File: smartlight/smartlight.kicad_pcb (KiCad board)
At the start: 2 copper layers, 43 x 37.5 mm, 22 parts, among them J1 Conn_01x06, J2 Conn_01x05, U1 ESP-12F

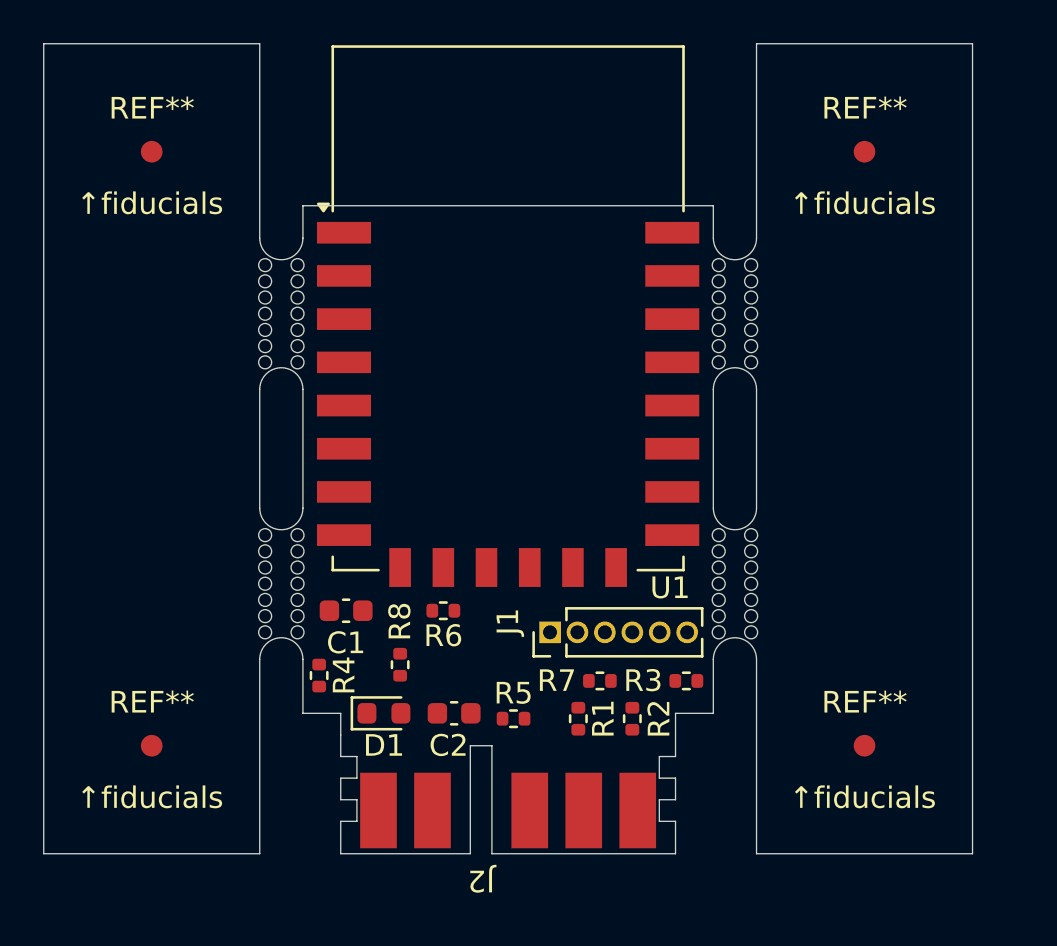
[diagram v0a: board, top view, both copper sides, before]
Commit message: before swapping pin snapshot
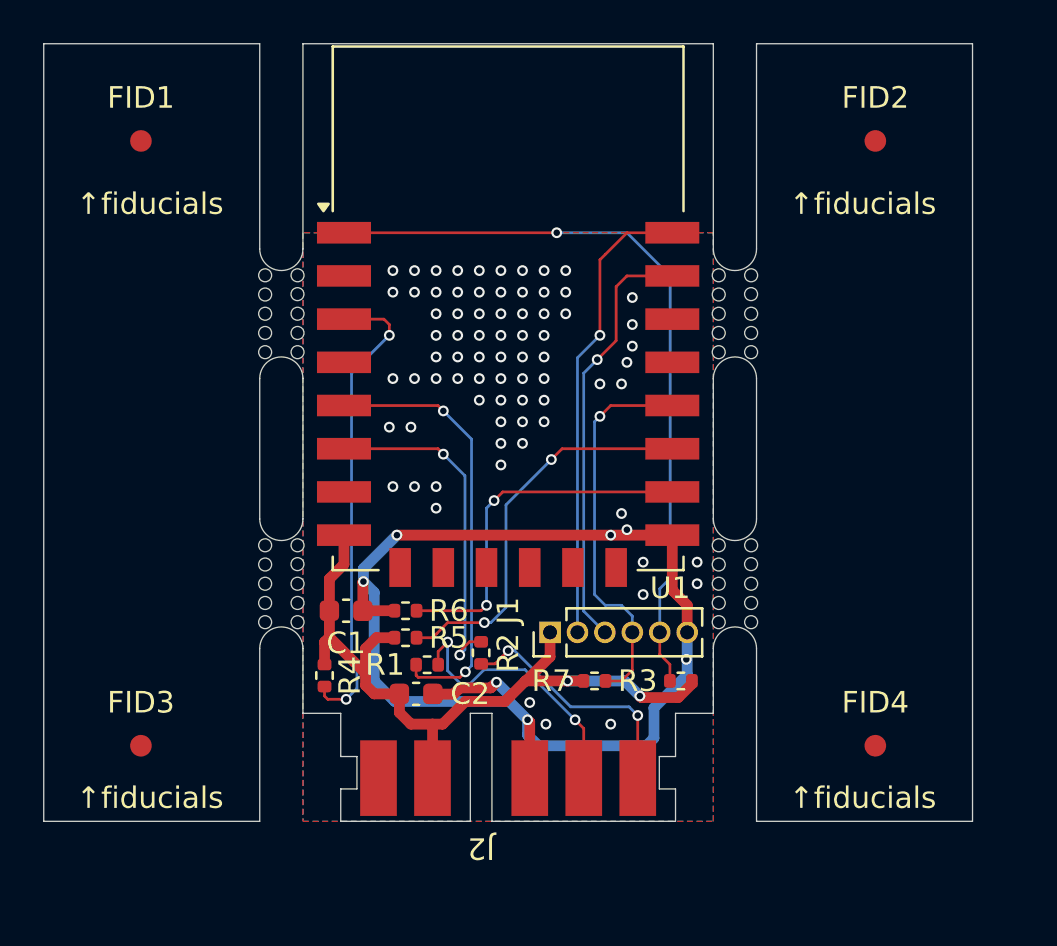
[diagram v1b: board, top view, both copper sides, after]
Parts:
- removed D1: LED, LED_SMD:LED_0603_1608Metric
- removed R8: 2k, Resistor_SMD:R_0402_1005Metric
- removed REF** (x4): mousebites_1mm, taki-library:mousebites_1mm
- removed REF** (x4): Fiducial_1mm_Mask2mm, Fiducial:Fiducial_1mm_Mask2mm
- added FID1: Fiducial, Fiducial:Fiducial_1mm_Mask2mm, F.Cu at (73.0, 42.0)
- added FID2: Fiducial, Fiducial:Fiducial_1mm_Mask2mm, F.Cu at (107.0, 42.0)
- added FID3: Fiducial, Fiducial:Fiducial_1mm_Mask2mm, F.Cu at (73.0, 70.0)
- added FID4: Fiducial, Fiducial:Fiducial_1mm_Mask2mm, F.Cu at (107.0, 70.0)
- added H1: mousebite, taki-library:mousebites_1mm, F.Cu at (79.5, 62.5)
- added H2: mousebite, taki-library:mousebites_1mm, F.Cu at (79.5, 50.0)
- added H3: mousebite, taki-library:mousebites_1mm, F.Cu at (100.5, 50.0)
- added H4: mousebite, taki-library:mousebites_1mm, F.Cu at (100.5, 62.5)
- moved R2 7.64 mm to (88.8, 65.7)
- moved R1 7.43 mm to (86.2, 66.2), turned to 0 degrees
- moved R5 6.25 mm to (85.2, 65.0)
- moved C2 1.98 mm to (85.7, 67.6)
- moved R6 1.75 mm to (85.2, 63.8)
- moved J2 1.50 mm to (91.0, 71.5)
- moved R3 0.25 mm to (98.0, 67.0)
- moved R4 0.25 mm to (81.5, 66.8)
- moved R7 0.25 mm to (94.0, 67.0)
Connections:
- U1 pad 20: Net-(U1-GPIO5) -> unconnected-(U1-GPIO5-Pad20)
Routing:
- net GND: track 0.00 -> 55.3 mm, vias 0 -> 82
- net +3V3: track 0.00 -> 35.9 mm, vias 0 -> 2
- net RESET: track 0.00 -> 35.1 mm, vias 0 -> 1
- net Net-(U1-EN): track 0.00 -> 22.1 mm, vias 0 -> 2
- net ESP12F_TX: track 0.00 -> 21.5 mm, vias 0 -> 1
- net PWM: track 0.00 -> 20.4 mm, vias 0 -> 2
- net ESP12F_RX: track 0.00 -> 19.8 mm, vias 0 -> 1
- net Net-(U1-GPIO2): track 0.00 -> 18.2 mm, vias 0 -> 2
- net IO0: track 0.00 -> 18.0 mm, vias 0 -> 1
- net Net-(U1-GPIO15): track 0.00 -> 16.8 mm, vias 0 -> 2
- net ON/OFF: track 0.00 -> 15.9 mm, vias 0 -> 2
- net Net-(J2-Pin_2): track 0.00 -> 15.7 mm, vias 0 -> 2
- net Net-(J2-Pin_1): track 0.00 -> 14.2 mm, vias 0 -> 2
- added copper zone on B.Cu, net GND
- added copper zone on F.Cu, net GND
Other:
- board size 43 x 37.5 mm -> 43 x 36 mm
